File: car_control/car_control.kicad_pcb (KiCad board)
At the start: 2 copper layers, 55.9 x 76.8 mm, 25 parts, among them J1 Conn_01x02, J2 Conn_01x03, J3 Conn_01x03, Q1 IRF540N, Q2 Q_Photo_NPN, SW1 SW_SPST

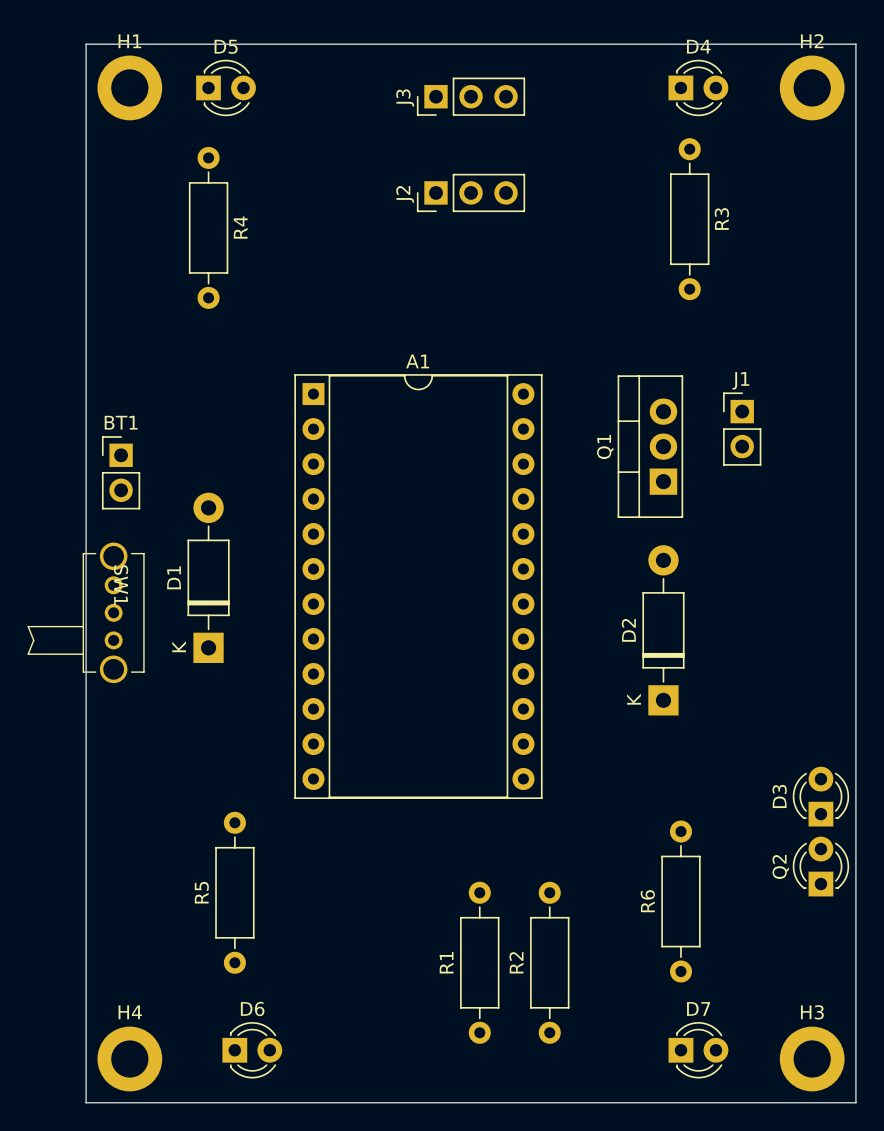
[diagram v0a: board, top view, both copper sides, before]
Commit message: working on mechanics
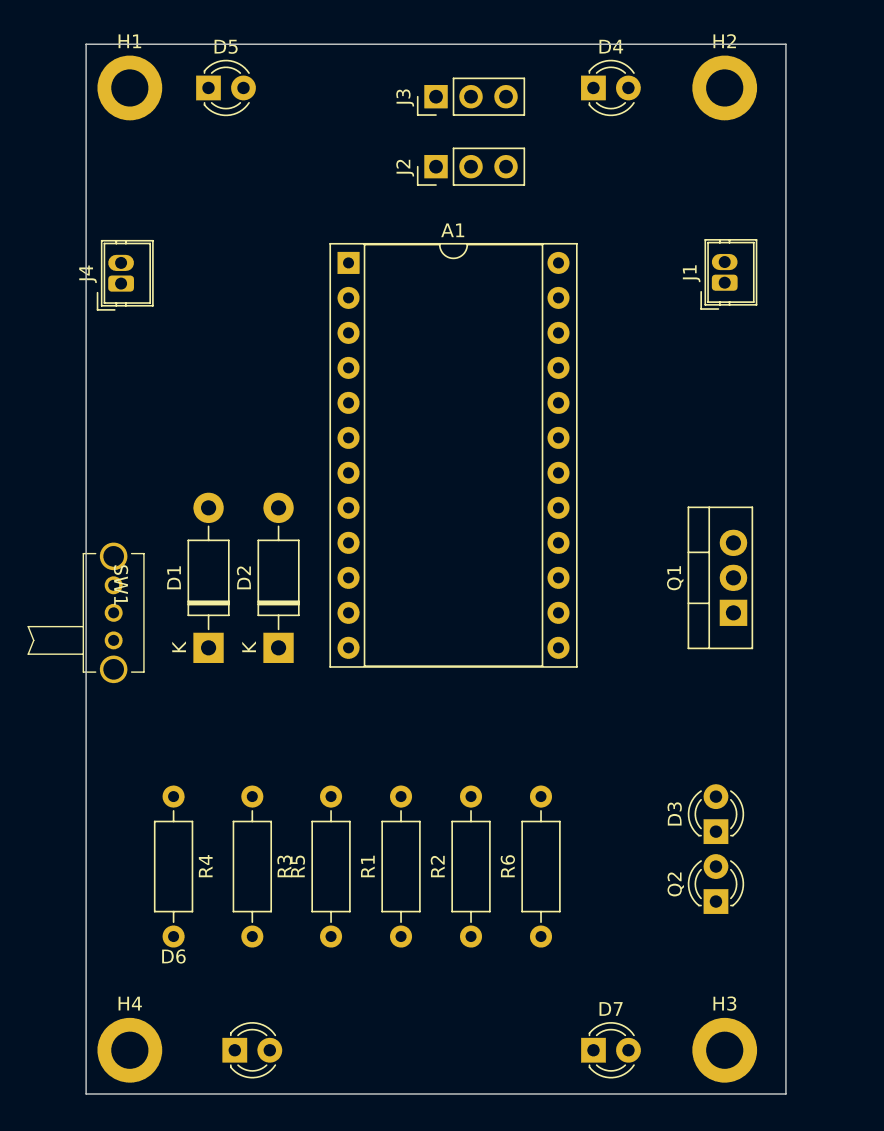
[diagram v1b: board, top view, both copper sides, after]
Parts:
- removed BT1: Battery, Connector_PinHeader_2.54mm:PinHeader_1x02_P2.54mm_Vertical
- added J4: Screw_Terminal_01x02, Connector_Wuerth:Wuerth_WR-WTB_64800211622_1x02_P1.50mm_Vertical, F.Cu at (134.6, 44.7)
- J1: value Conn_01x02 -> Screw_Terminal_01x02; footprint Connector_PinHeader_2.54mm:PinHeader_1x02_P2.54mm_Vertical -> Connector_Wuerth:Wuerth_WR-WTB_64800211622_1x02_P1.50mm_Vertical
- moved R3 56.7 mm to (144.1, 81.9)
- moved R4 46.4 mm to (138.4, 81.9)
- moved D2 28.2 mm to (146.1, 71.1)
- moved Q1 10.8 mm to (179.1, 68.6)
- moved R6 10.5 mm to (165.1, 92.1)
- moved A1 9.85 mm to (151.1, 43.2)
- moved J1 9.44 mm to (178.4, 44.6), turned to 90 degrees
- moved R1 9.03 mm to (154.9, 92.1)
- moved R2 9.03 mm to (160.0, 92.1)
- moved D3 7.73 mm to (177.8, 84.5)
- moved Q2 7.73 mm to (177.8, 89.5)
- moved R5 7.24 mm to (149.9, 92.1)
- moved H3 6.38 mm to (178.4, 100.3)
- moved D4 6.35 mm to (168.9, 30.5)
- moved D7 6.35 mm to (168.9, 100.3)
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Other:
- board size 55.9 x 76.8 mm -> 50.8 x 76.2 mm
